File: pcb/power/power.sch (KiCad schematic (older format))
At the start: 57 parts, among them CON1 BARREL_JACK, P1 CONN_01X04, P2 CONN_01X04, P3 CONN_01X04, P4 USB_A, P5 CONN_01X03, P6 CONN_01X03, U1 TS30012, U2 LM324QT, U3 LM2840

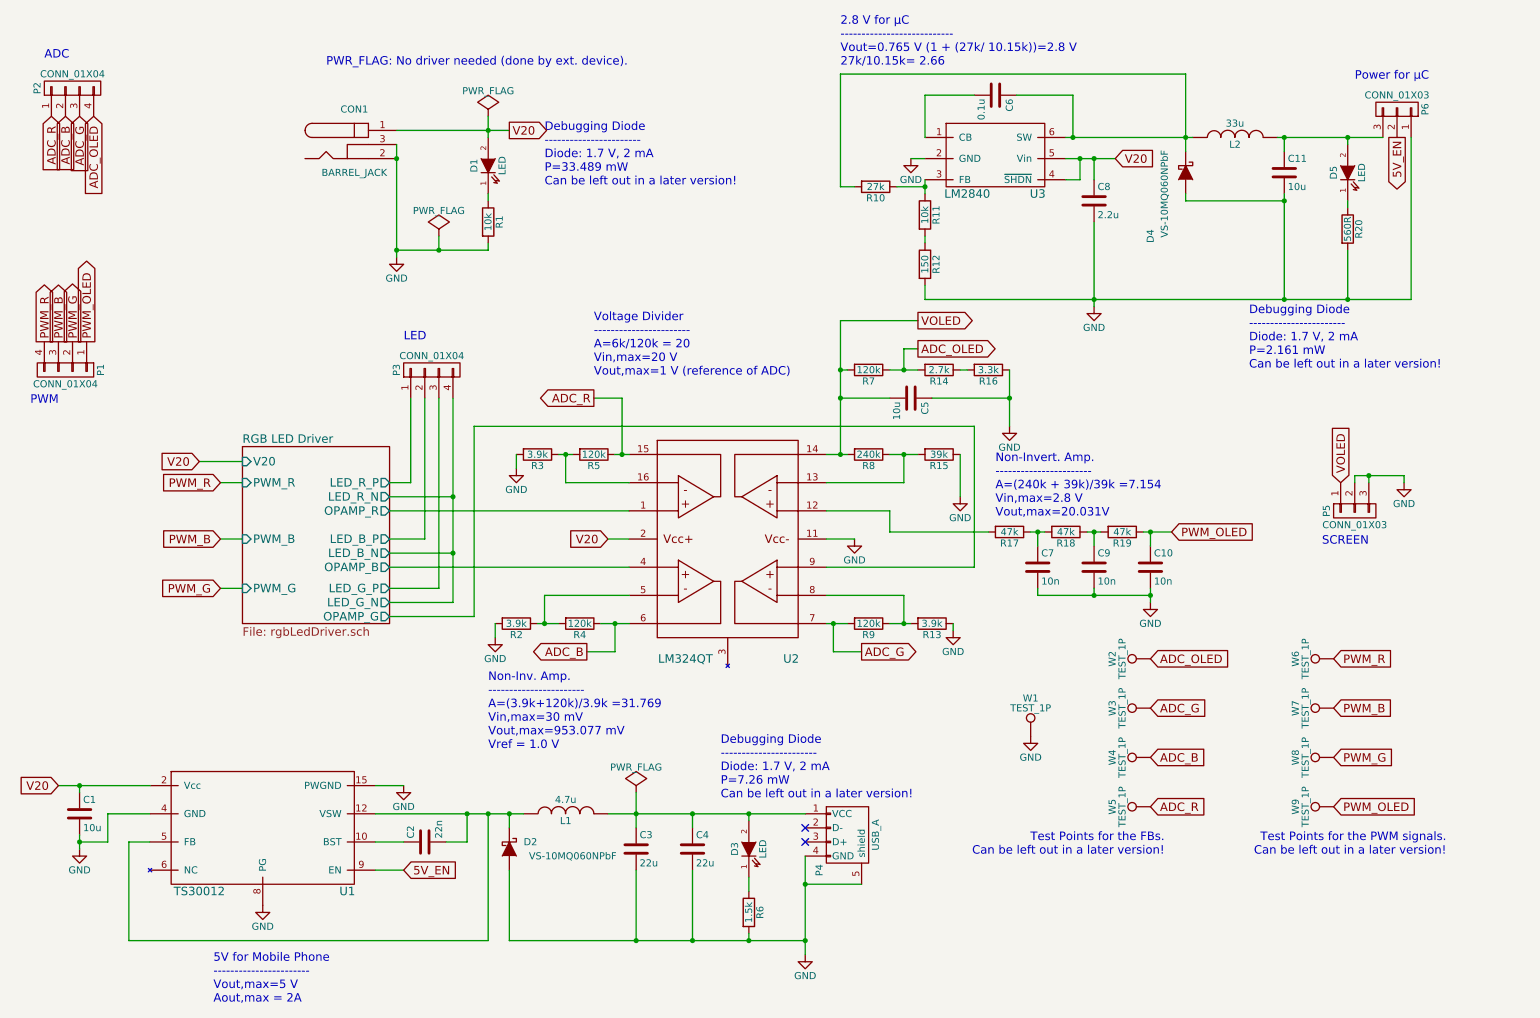
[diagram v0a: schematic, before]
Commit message: Finished the schematics.
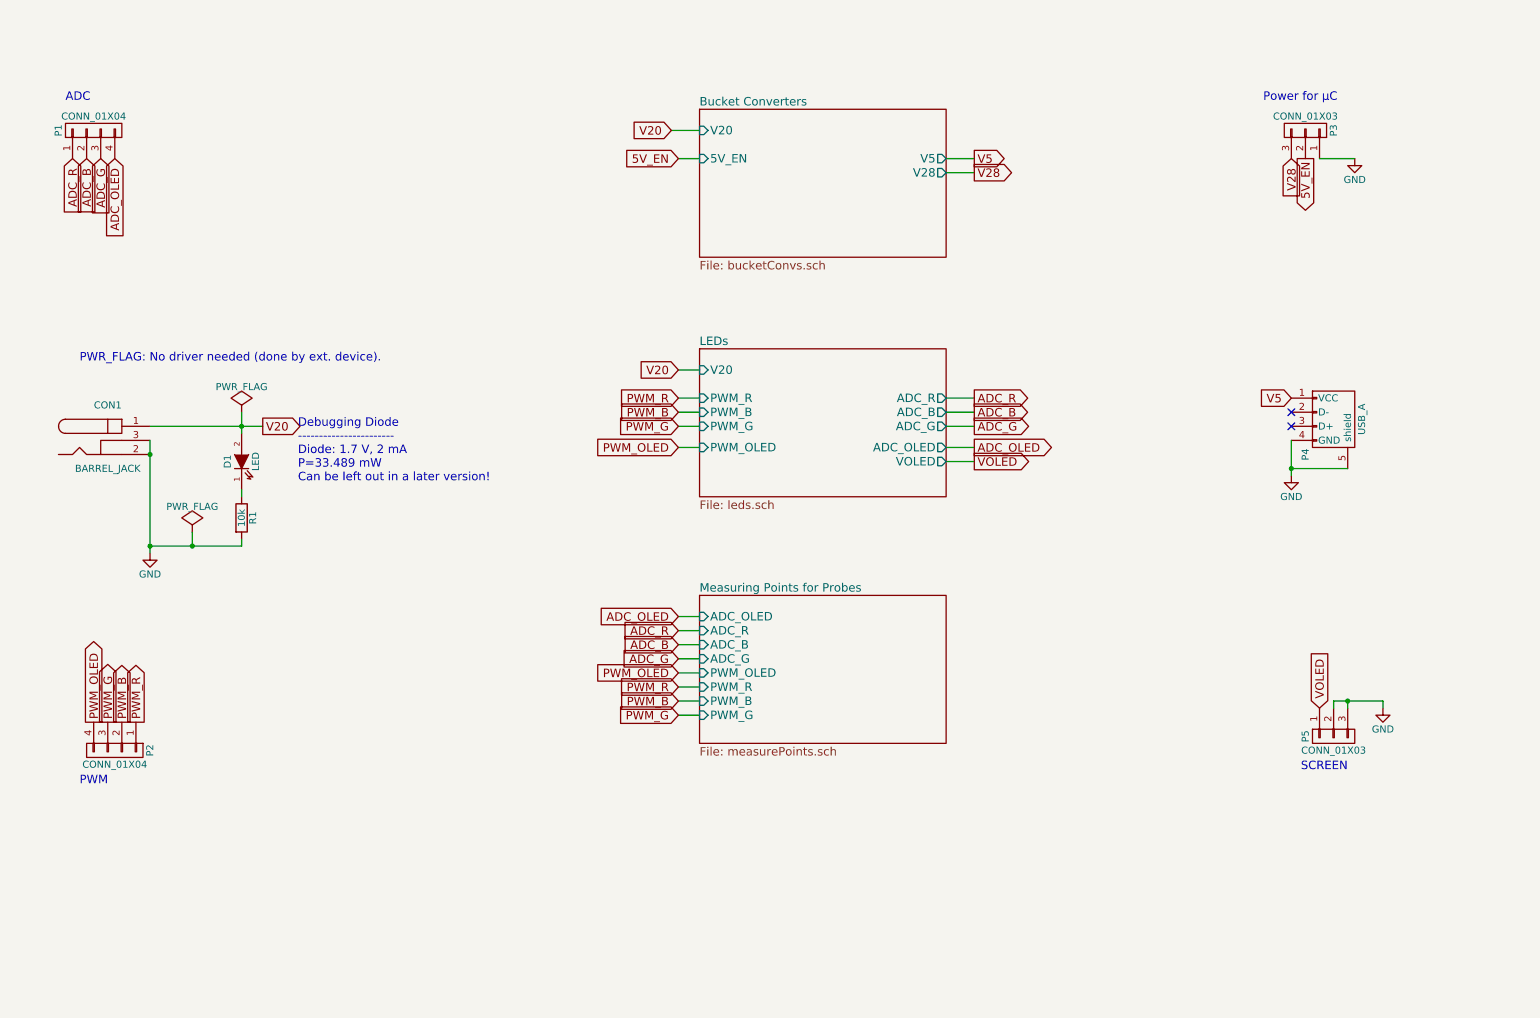
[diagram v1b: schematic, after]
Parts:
- removed C1, C11, C5: 10u, Capacitors_SMD:C_0603_HandSoldering, symbol C
- removed C10, C7, C9: 10n, Capacitors_SMD:C_0603_HandSoldering, symbol C
- removed C2: 22n, Capacitors_SMD:C_0603_HandSoldering, symbol C
- removed C3, C4: 22u, Capacitors_SMD:C_0603_HandSoldering, symbol C
- removed C6: 0.1u, Capacitors_SMD:C_0603_HandSoldering, symbol C
- removed C8: 2.2u, Capacitors_SMD:C_0603_HandSoldering, symbol C
- removed D2, D4: VS-10MQ060NPbF, Diodes_SMD:SMA_Handsoldering, symbol D_Schottky
- removed D3, D5: LED, LEDs:LED_0603, symbol LED
- removed L1: 4.7u, Additional:Taiyo_Yuden_NRS8030_IND, symbol INDUCTOR
- removed L2: 33u, Additional:Bourns_SRN3015, symbol INDUCTOR
- removed P3: CONN_01X04, Connect:PINHEAD1-3, symbol CONN_01X04
- removed P6: CONN_01X03, Pin_Headers:Pin_Header_Straight_1x03, symbol CONN_01X03
- removed R10: 27k, Resistors_SMD:R_0603_HandSoldering, symbol R
- removed R11: 10k, Resistors_SMD:R_0603_HandSoldering, symbol R
- removed R12: 150, Resistors_SMD:R_0603_HandSoldering, symbol R
- removed R13, R2, R3: 3.9k, Resistors_SMD:R_0603_HandSoldering, symbol R
- removed R14: 2.7k, Resistors_SMD:R_0603_HandSoldering, symbol R
- removed R15: 39k, Resistors_SMD:R_0603_HandSoldering, symbol R
- removed R16: 3.3k, Resistors_SMD:R_0603_HandSoldering, symbol R
- removed R17, R18, R19: 47k, Resistors_SMD:R_0603_HandSoldering, symbol R
- removed R20: 560R, Resistors_SMD:R_0603_HandSoldering, symbol R
- removed R4, R5, R7, R9: 120k, Resistors_SMD:R_0603_HandSoldering, symbol R
- removed R6: 1.5k, Capacitors_SMD:C_0603_HandSoldering, symbol R
- removed R8: 240k, Resistors_SMD:R_0603_HandSoldering, symbol R
- removed U1: TS30012, Additional:QFN-16-1EP_3x3mm_Pitch0.5mm, symbol TS30012
- removed U2: LM324QT, Additional:QFN-16-1EP_3x3mm_Pitch0.5mm, symbol LM324QT
- removed U3: LM2840, TO_SOT_Packages_SMD:SOT-23-6, symbol LM2840
- removed W1: TEST_1P, Measurement_Points:Measurement_Point_Round-SMD-Pad_Big, symbol TEST_1P
- removed W2, W3, W4, W5, W6, W7, W8, W9: TEST_1P, Additional:TP_PROBE, symbol TEST_1P
- added P3: CONN_01X03, Pin_Headers:Pin_Header_Straight_1x03, symbol CONN_01X03
- renumbered P2 to P1, P1 to P2
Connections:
- net 5V_EN: now also P3.2 (P2)
- net GND: now also P3.1 (P1)
- net PWM_B: now also P2.2 (P2); no longer P2.3 (P3)
- net PWM_G: now also P2.3 (P3); no longer P2.2 (P2)
- net PWM_OLED: now also P2.4 (P4); no longer P2.1 (P1)
- net PWM_R: now also P2.1 (P1); no longer P2.4 (P4)
- net V5: now reaches P4.1 (VCC)
- net Vcc renamed V20
- new net V28: P3.3 (P3)
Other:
- note removed: "2.8 V for µC\n---------------------------\nVout=0.765 V (1 + (27k/ 10.15k))=2.8 V\n27k/10.15k= 2.66"
- note removed: "5V for Mobile Phone\n-----------------------\nVout,max=5 V\nAout,max = 2A"
- note removed: "Debugging Diode\n-----------------------\nDiode: 1.7 V, 2 mA\nP=2.161 mW\nCan be left out in a later version!"
- note removed: "Debugging Diode\n-----------------------\nDiode: 1.7 V, 2 mA\nP=7.26 mW\nCan be left out in a later version!"
- note removed: "LED"
- note removed: "Non-Inv. Amp.\n-----------------------\nA=(3.9k+120k)/3.9k =31.769\nVin,max=30 mV\nVout,max=953.077 mV\nVref = 1.0 V"
- note removed: "Non-Invert. Amp.\n-----------------------\nA=(240k + 39k)/39k =7.154\nVin,max=2.8 V\nVout,max=20.031V"
- note removed: "Test Points for the FBs.\nCan be left out in a later version!"
- note removed: "Test Points for the PWM signals.\nCan be left out in a later version!"
- note removed: "Voltage Divider\n-----------------------\nA=6k/120k = 20\nVin,max=20 V\nVout,max=1 V (reference of ADC)"
- moved on the sheet: CON1, D1, P1, P2, P5, R1
